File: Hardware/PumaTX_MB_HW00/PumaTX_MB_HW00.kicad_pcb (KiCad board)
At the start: 4 copper layers, 130 x 40 mm, 110 parts, among them J100 FH12A-26S-0.5SH_55_, J101 FH12-12S-0.5SH_55_, J102 500334-0160, J103 500334-0160, J104 692122030100, J105 53398-0667, J400 U.FL-R-SMT-1_40_, J410 U.FL-R-SMT-1_40_, M130 Motor_DC, M140 Fan, Q130 ZXMN3B01F, Q140 ZXMN3B01F, Q200 UMH3NTN, Q201 UMH3NTN, U200 CP2105-F01-GMR, U300 ESP32-PICO-D4, U400 ESP32-PICO-D4, U402 E28-2G4M27S, U410 SX1280, U500 BQ24075RGTR, U510 MIC5528-3.3YMT-T5, U520 MIC5528-3.3YMT-T5, U530 MIC5528-3.3YMT-T5, Y410 NX2016SA-52MHZ-EXS00A-CS06016

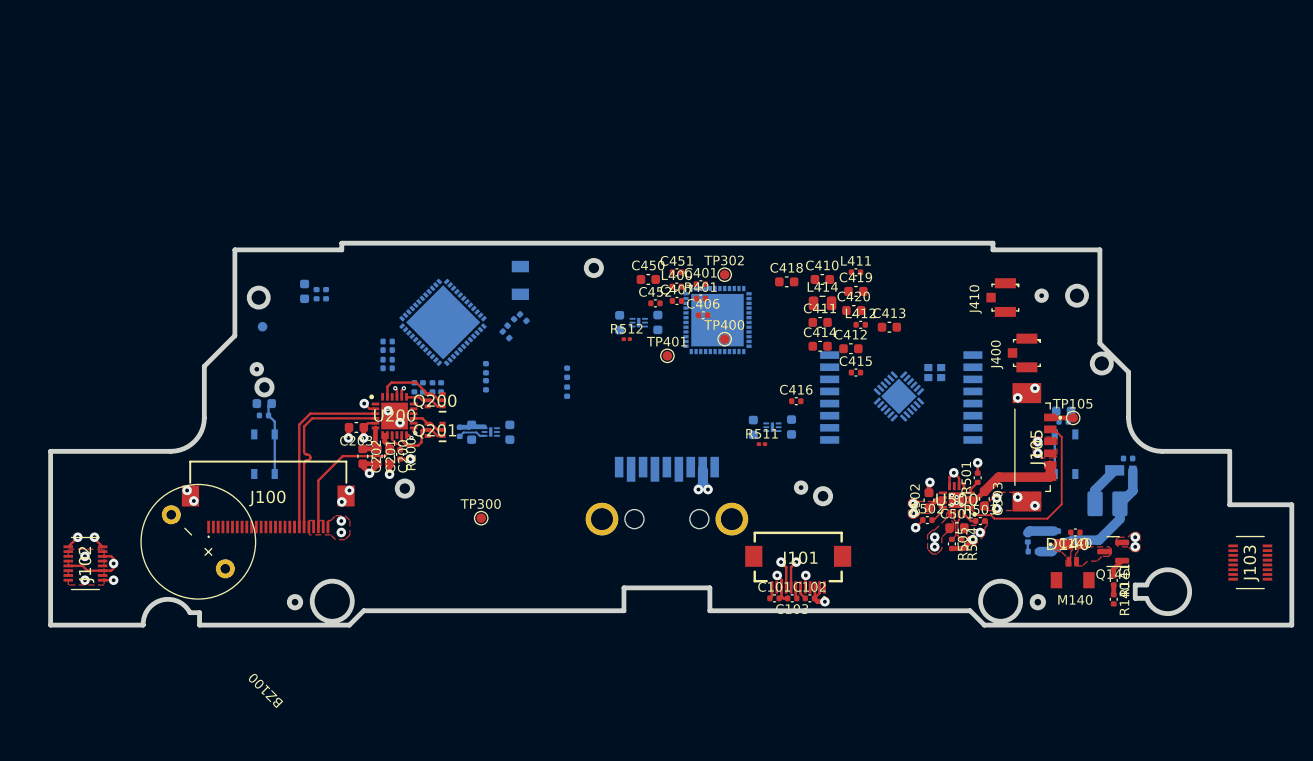
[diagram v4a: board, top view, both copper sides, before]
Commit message: Routing update
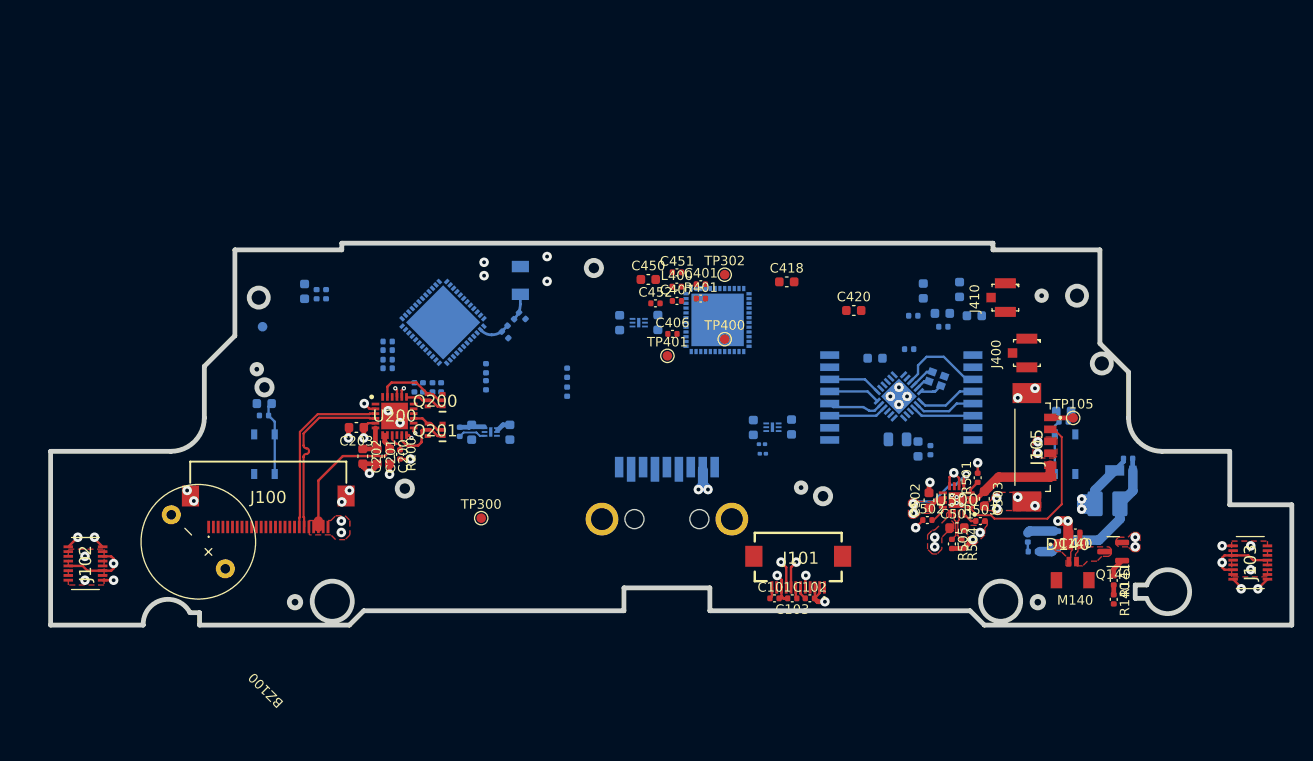
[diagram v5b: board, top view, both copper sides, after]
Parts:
- C410, C411, C412, C413, C414, C415, C416, C419, L411, L412, L414, R511, R512: moved to B.Cu
- moved R512 18.6 mm to (156.0, 105.2), turned to 180 degrees
- moved C419 17.7 mm to (172.2, 104.8), turned to -90 degrees
- moved L414 16.3 mm to (170.1, 103.8), turned to 180 degrees
- moved C416 15.0 mm to (173.6, 104.9), turned to -90 degrees
- moved C414 13.3 mm to (174.8, 90.5)
- moved C412 13.0 mm to (176.6, 88.0), turned to 90 degrees
- moved C411 11.3 mm to (172.8, 88.2), turned to 90 degrees
- moved C410 9.93 mm to (167.8, 95.2), turned to 180 degrees
- moved C413 8.98 mm to (178.2, 90.8)
- moved L412 8.65 mm to (174.9, 92.0)
- moved L411 7.53 mm to (171.8, 90.8)
- moved C415 6.09 mm to (171.3, 94.3)
- moved C406 3.76 mm to (146.5, 92.7)
- moved Y410 0.68 mm to (174.2, 97.4), turned to 160 degrees
- moved C307 0.22 mm to (130.8, 90.8)
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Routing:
- net /VSYS: track 8.96 -> 52.3 mm, vias 2 -> 7
- net /NRESET: track 0.00 -> 9.13 mm
- net +3V3: track 12.2 -> 21.0 mm, vias 3 -> 4
- net /DIO2: track 0.00 -> 6.53 mm
- net /DIO1: track 0.00 -> 6.46 mm
- net /MISO: track 0.00 -> 6.03 mm
- net /MOSI: track 0.00 -> 5.87 mm
- net /BUSY: track 0.00 -> 5.82 mm
- net /NSS: track 0.00 -> 5.52 mm
- net /SCK: track 0.00 -> 5.41 mm
- net /50_PUMATX_ANT_1: track 0.00 -> 3.31 mm
- net /50_PUMATX_ANT_2: track 0.18 -> 2.95 mm
- net /C2: track 4.15 -> 6.88 mm
- net /XTA: track 0.00 -> 2.51 mm
- net /XTB: track 0.00 -> 2.40 mm
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- added copper zone on In2.Cu, net GND
